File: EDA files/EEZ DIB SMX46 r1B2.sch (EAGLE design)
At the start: 156 parts, among them IC1 STM32F030C6T6, IC2 74HC1G126GW,125, IC3 M24C32-WMN6P, IC4 LP2985-33DBVR, IC5 74HC2G04GW,125, IC6 OPA2170, K1 FTR-C1GA012G-B05, K10 FTR-C1GA012G-B05, K11 FTR-C1GA012G-B05, K12 FTR-C1GA012G-B05, K13 FTR-C1GA012G-B05, K14 FTR-C1GA012G-B05, K15 FTR-C1GA012G-B05, K16 FTR-C1GA012G-B05, K17 FTR-C1GA012G-B05, K18 FTR-C1GA012G-B05, K19 FTR-C1GA012G-B05, K2 FTR-C1GA012G-B05, K20 FTR-C1GA012G-B05, K21 FTR-C1GA012G-B05, K22 FTR-C1GA012G-B05, K23 FTR-C1GA012G-B05, K24 FTR-C1GA012G-B05, K3 FTR-C1GA012G-B05, K4 FTR-C1GA012G-B05, K5 FTR-C1GA012G-B05, K6 FTR-C1GA012G-B05, K7 FTR-C1GA012G-B05, K8 FTR-C1GA012G-B05, K9 FTR-C1GA012G-B05, Q1 2N7002, Q10 2N7002, Q11 2N7002, Q12 2N7002, Q13 2N7002, Q14 2N7002, Q15 2N7002, Q16 2N7002, Q17 2N7002, Q18 2N7002, Q19 2N7002, Q2 2N7002, Q20 2N7002, Q21 2N7002, Q22 2N7002, Q23 2N7002, Q24 2N7002, Q25 2N7002, Q3 2N7002, Q4 2N7002, Q5 2N7002, Q6 2N7002, Q7 2N7002, Q8 2N7002, Q9 2N7002, X1 SSW-106-02-S-S, X2 77317-104-28LF, X3 691327310016, X4 691327310016

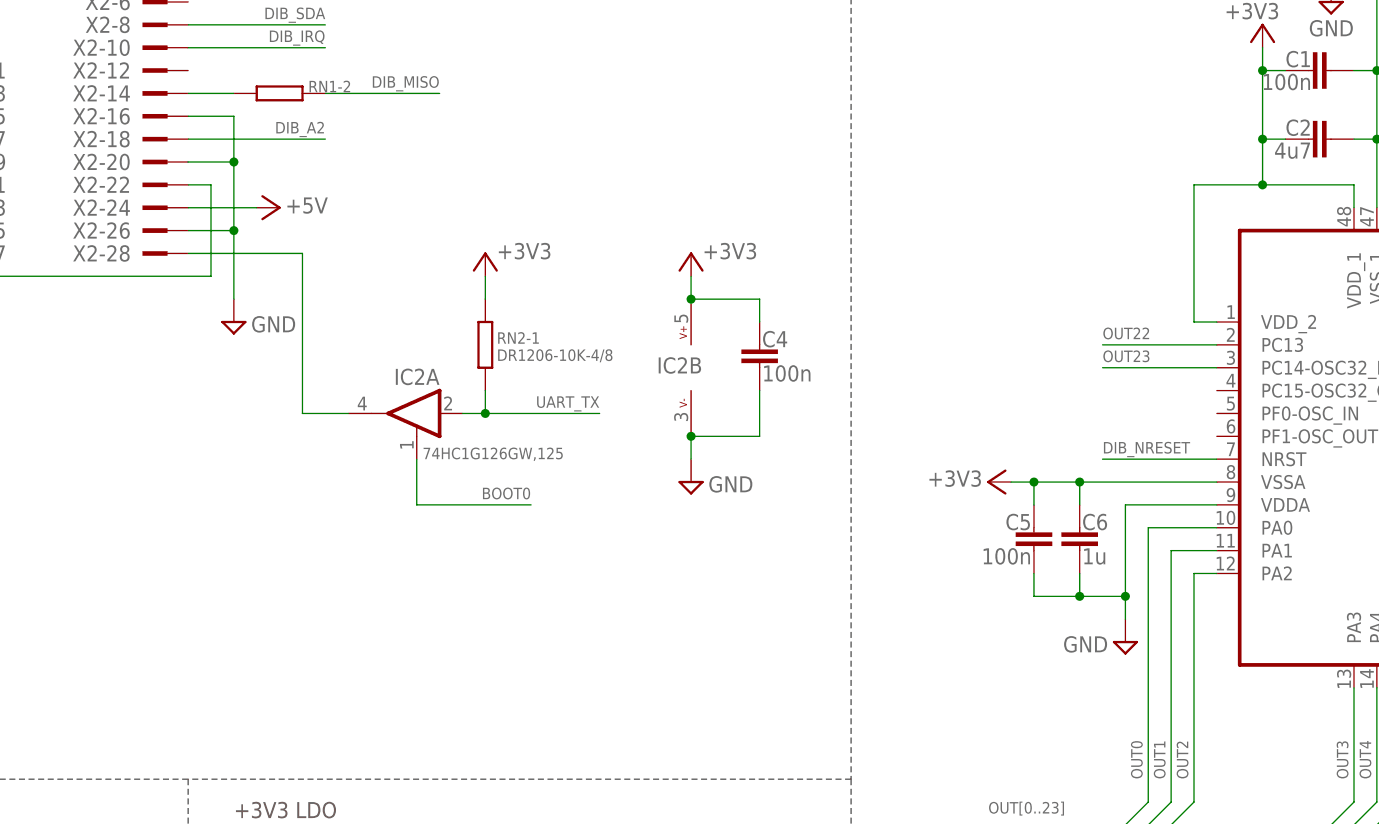
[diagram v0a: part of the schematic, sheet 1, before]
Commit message: #1, #2 fixed
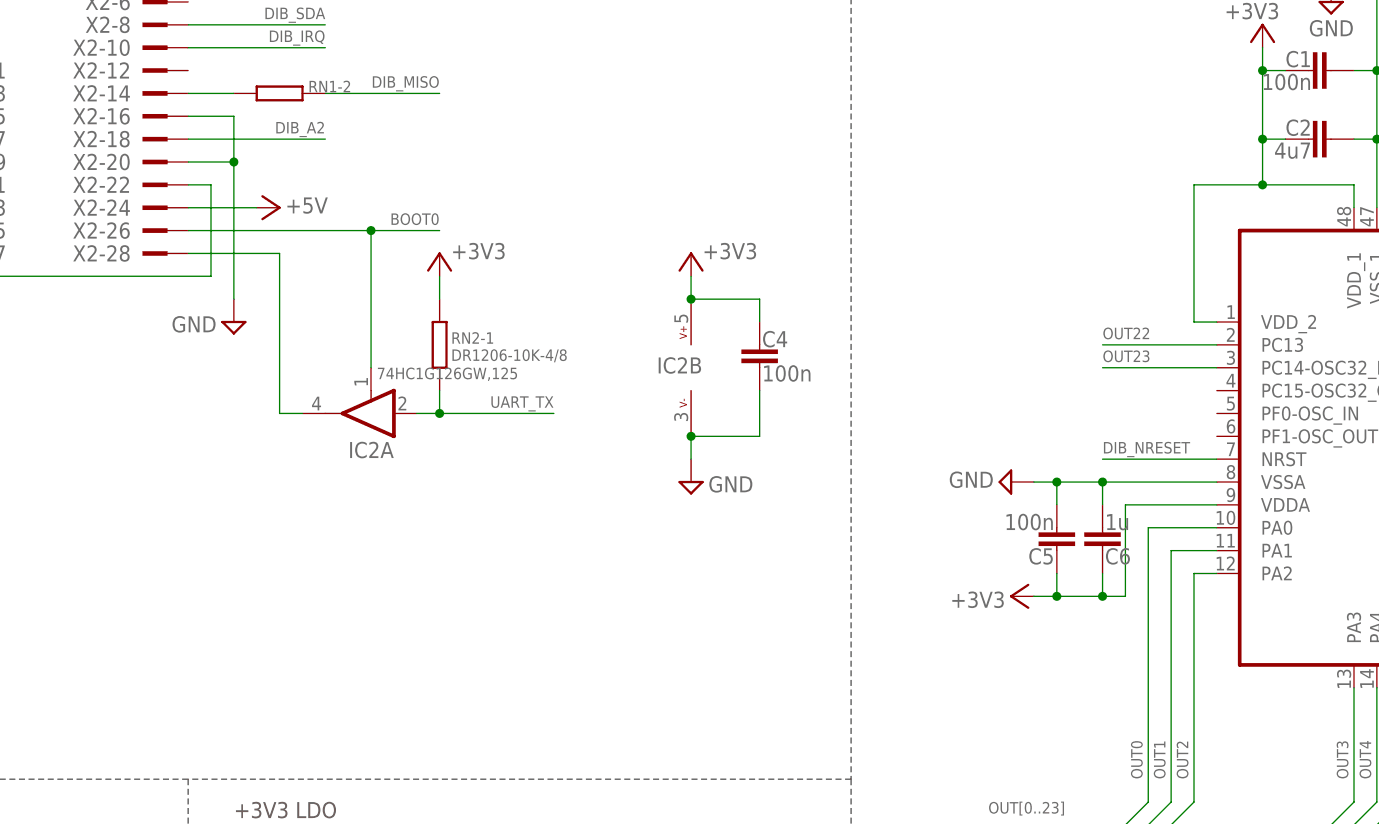
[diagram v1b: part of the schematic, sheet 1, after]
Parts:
- C2, C9: device rcl:C-EUC1206 -> rcl:C-EUC0805
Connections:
- net +3V3: now also IC1.VDDA; no longer IC1.VSSA
- net BOOT0: now also X2-26.1
- net GND: now also IC1.VSSA; no longer IC1.VDDA, X2-26.1
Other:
- moved on the sheet: C5, C6, IC2A, RN2-1
